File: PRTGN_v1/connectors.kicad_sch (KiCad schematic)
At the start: 10 parts, among them J3 Conn_02x08_Odd_Even, J5 USB_TypeC, M1 Fan_4pin, M2 Fan_4pin, U2 USBLC6-2SC6

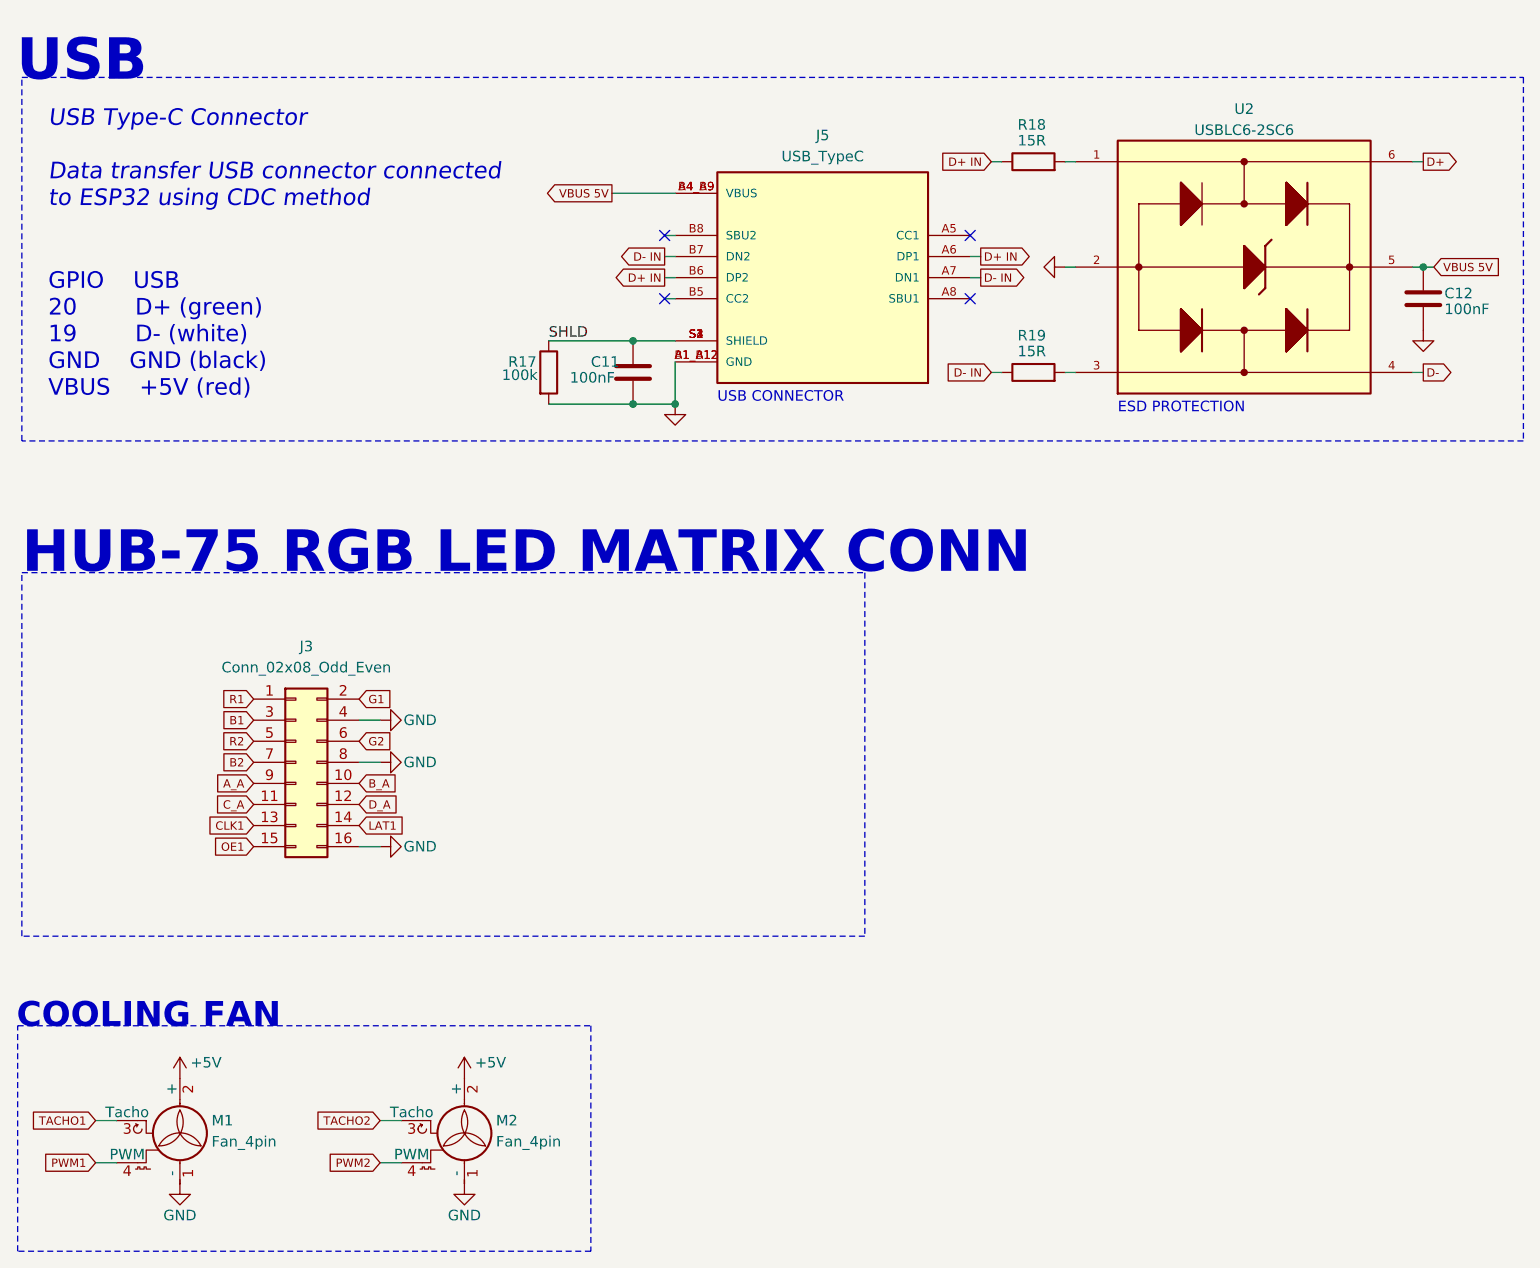
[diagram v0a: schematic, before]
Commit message: upd
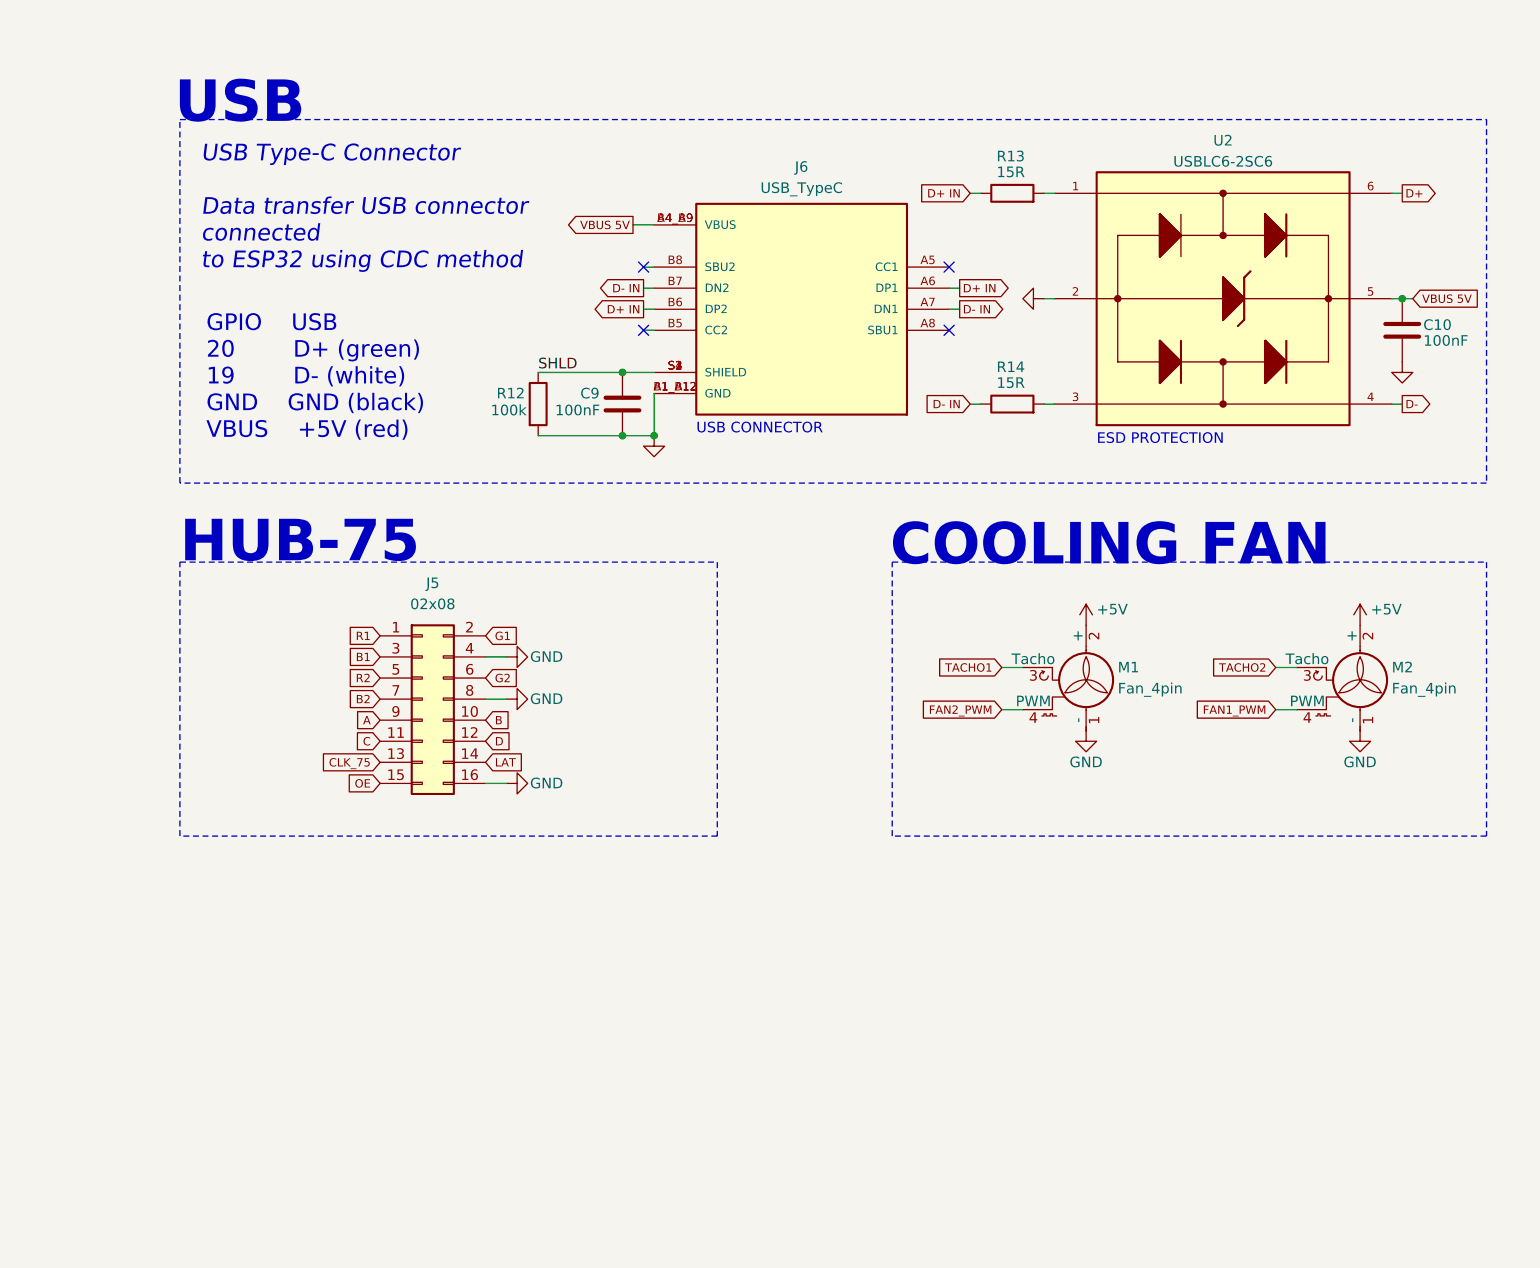
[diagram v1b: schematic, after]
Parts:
- J5: renamed from J3; value Conn_02x08_Odd_Even -> 02x08
- renumbered C12 to C10, C11 to C9, J5 to J6, R17 to R12, R18 to R13, R19 to R14
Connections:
- net A_A renamed A
- net B_A renamed B
- net CLK1 renamed CLK_75
- net C_A renamed C
- net D_A renamed D
- net LAT1 renamed LAT
- net OE1 renamed OE
- net PWM1 renamed FAN2_PWM
- net PWM2 renamed FAN1_PWM
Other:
- note added: "HUB-75"
- note removed: "HUB-75 RGB LED MATRIX CONN"
- moved on the sheet: C10, C9, J5, J6, M1, M2, R12, R13, R14, U2
